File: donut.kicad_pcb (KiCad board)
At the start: 2 copper layers, 78.5 x 68.9 mm, 47 parts, among them J1 AVRISP6, J2 Jack, J3 HALL2, P1 PAD1, P2 PAD2, SW1 S0, SW10 TACTILE, SW11 TACTILE, SW12 TACTILE, SW13 MODE, SW2 TACTILE, SW3 TACTILE, SW4 TACTILE, SW5 TACTILE, SW6 TACTILE, SW7 TACTILE, SW8 TACTILE, SW9 TACTILE, U1 ATMEGA48PA-MU, X1 XTAL4P

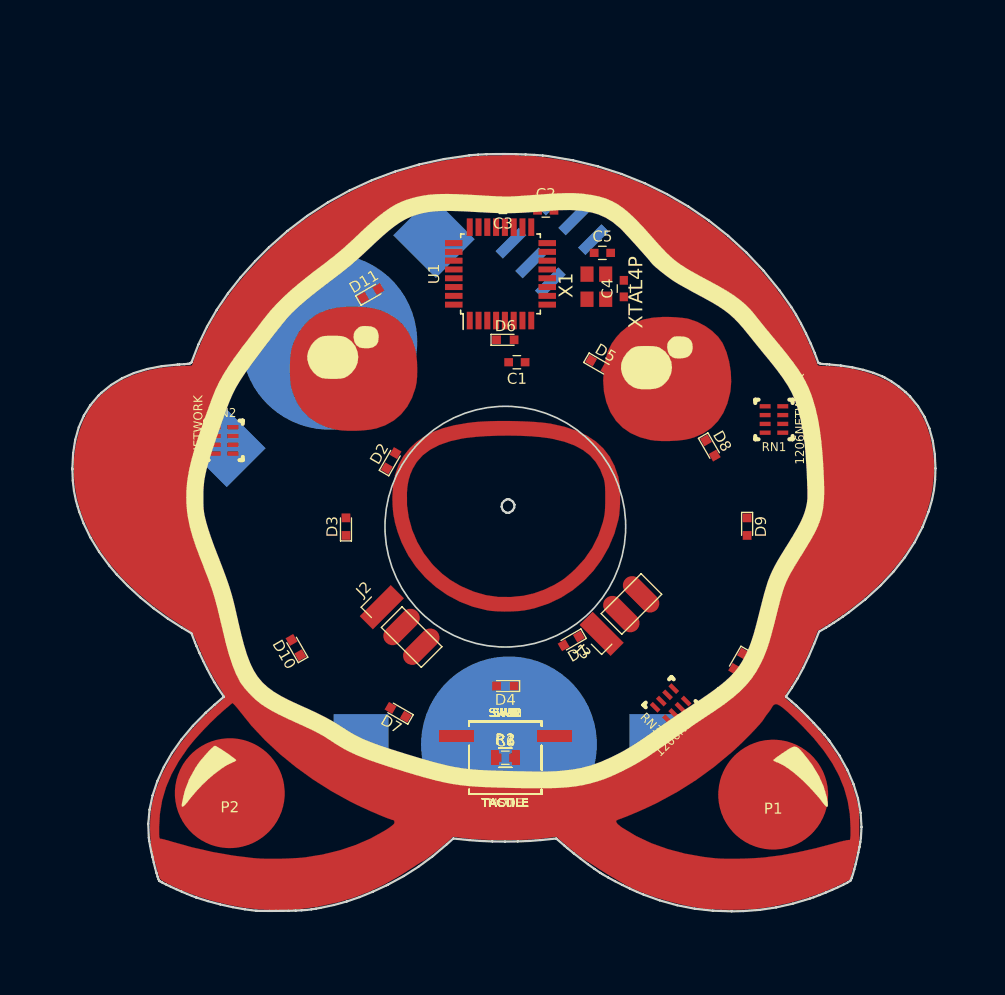
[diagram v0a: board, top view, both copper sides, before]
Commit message: Update donut
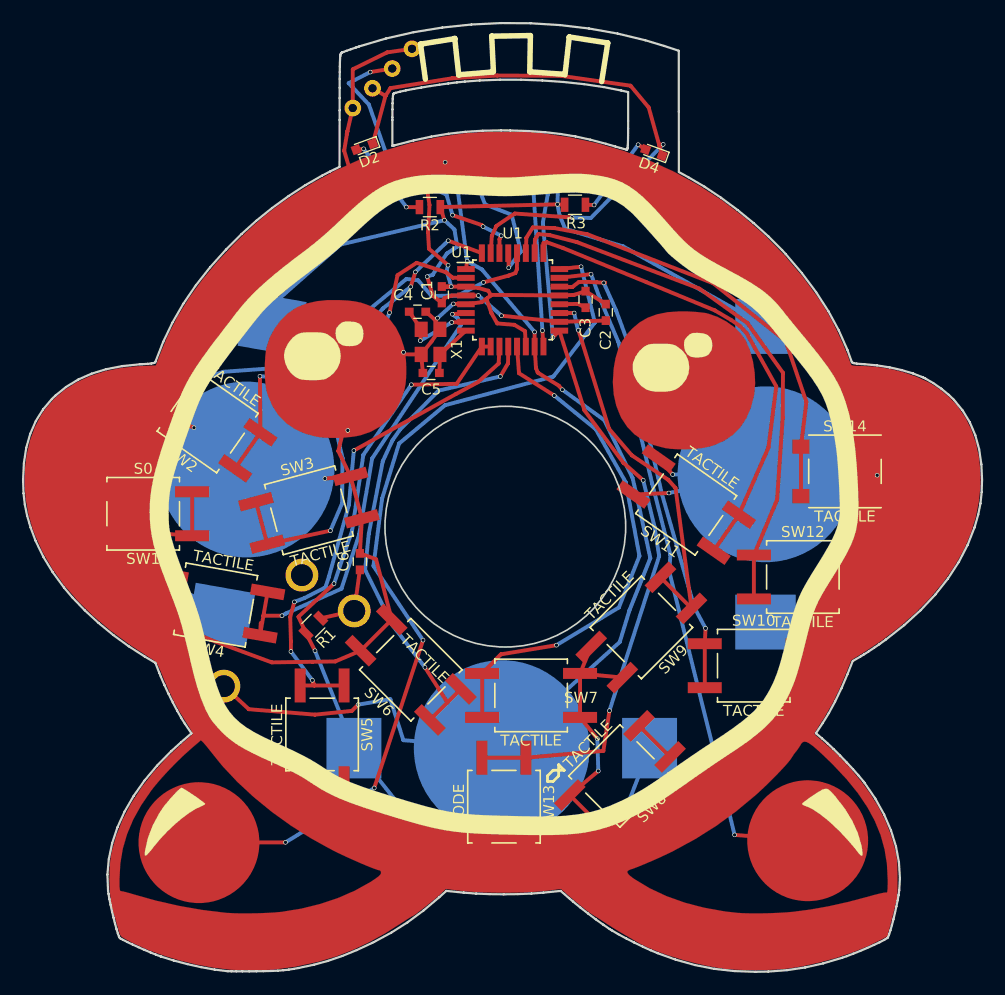
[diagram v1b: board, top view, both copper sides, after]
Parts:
- removed D1, D11, D3, D5, D7, D9: GRN, LED_0603
- removed D10, D12, D6, D8: RED, LED_0603
- removed G***: LOGO, kingdonut:kingdonut2
- removed J3: HALL2, Pin_Header_Straight_1x03_Pitch2.54mm
- removed RN1, RN2, RN3: 1206NETWORK, 1206NETWORK
- added BT2: Battery_Cell, S8211-45R, B.Cu at (-23.6, -5.20)
- added G0: PAD1, kingdonut2, F.Cu at (-0.21, -5.97)
- added P3: PAD2, SMTPIN, F.Cu at (-8.49, -43.5)
- added P4: PAD1, SMTPIN, F.Cu at (-10.3, -41.7)
- added P5: PAD2, SMTPIN, F.Cu at (-12.1, -39.9)
- added P6: PAD2, SMTPIN, F.Cu at (-13.9, -38.1)
- added SW14: TACTILE, TACTILE10Small, F.Cu at (30.9, -5.03)
- C3: value .1uF -> .33uF
- J1: footprint RIBBON6SMT -> RIBBON6SMT_POGO
- J2: footprint Pin_Header_Straight_1x03_Pitch2.54mm -> 3.5mm_barrel_jack_MJ-3536N; moved to B.Cu
- moved R3 50.7 mm to (6.34, -29.3)
- moved R2 50.6 mm to (-6.87, -29.1), turned to 180 degrees
- moved D4 50.4 mm to (13.5, -34.0), turned to 160 degrees
- moved SW2 40.8 mm to (-27.1, -9.49), turned to 145 degrees
- moved LS1 40.2 mm to (-0.33, 20.1), turned to 0 degrees
- moved SW1 39.7 mm to (-33.0, -1.18), turned to 180 degrees
- moved BT1 33.9 mm to (23.7, -4.77), turned to 90 degrees
- moved SW12 31.7 mm to (27.1, 4.58)
- moved SW4 29.8 mm to (-26.4, 7.13), turned to 170 degrees
- moved SW3 28.7 mm to (-17.9, -1.49), turned to 15 degrees
- moved D2 28.7 mm to (-12.8, -34.6), turned to 200 degrees
- moved SW11 28.3 mm to (16.5, -2.00), turned to 145 degrees
- moved SW10 24.1 mm to (22.6, 12.7)
- moved C6 22.2 mm to (-13.2, 3.18), turned to 90 degrees
- moved R1 21.2 mm to (-17.5, 9.01), turned to 225 degrees
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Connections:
- U1 pad 11: TSW9 -> TSW4
- U1 pad 12: TSW7 -> TSW5
- U1 pad 13: TSW5 -> TSW6
- U1 pad 19: TSW10 -> TSW8
- U1 pad 2: TSW6 -> TSW2
- U1 pad 22: TSW11 -> TSW9
- U1 pad 25: TSW0 -> TSW10
- U1 pad 26: TSW1 -> TSW11
- U1 pad 27: TSW2 -> TSW12
- U1 pad 28: TSW3 -> TSW0
- U1 pad 30: (no net) -> RX
- U1 pad 32: TSW4 -> TSW1
- U1 pad 6: VCC -> TSW3
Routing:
- net GND: track 0.00 -> 335.4 mm, vias 0 -> 14
- net VCC: track 0.00 -> 165.8 mm, vias 0 -> 5
- net AUD-: track 0.00 -> 98.7 mm, vias 0 -> 4
- net AUD: track 0.00 -> 81.1 mm, vias 0 -> 3
- net Net-(P2-Pad1): track 0.00 -> 80.1 mm, vias 0 -> 4
- net SCK: track 0.00 -> 72.9 mm, vias 0 -> 3
- net Net-(P1-Pad1): track 0.00 -> 62.4 mm, vias 0 -> 2
- net TSW0: track 0.00 -> 57.9 mm, vias 0 -> 2
- net TX: track 0.00 -> 57.1 mm, vias 0 -> 2
- net TSW11: track 0.00 -> 49.3 mm
- net TSW6: track 0.00 -> 46.7 mm, vias 0 -> 2
- net TSW5: track 0.00 -> 45.2 mm, vias 0 -> 2
- net TSW4: track 0.00 -> 45.2 mm, vias 0 -> 4
- net TSW2: track 0.00 -> 43.4 mm, vias 0 -> 2
- net TSW10: track 0.00 -> 43.1 mm
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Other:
- board size 78.5 x 68.9 mm -> 87.3 x 86.3 mm

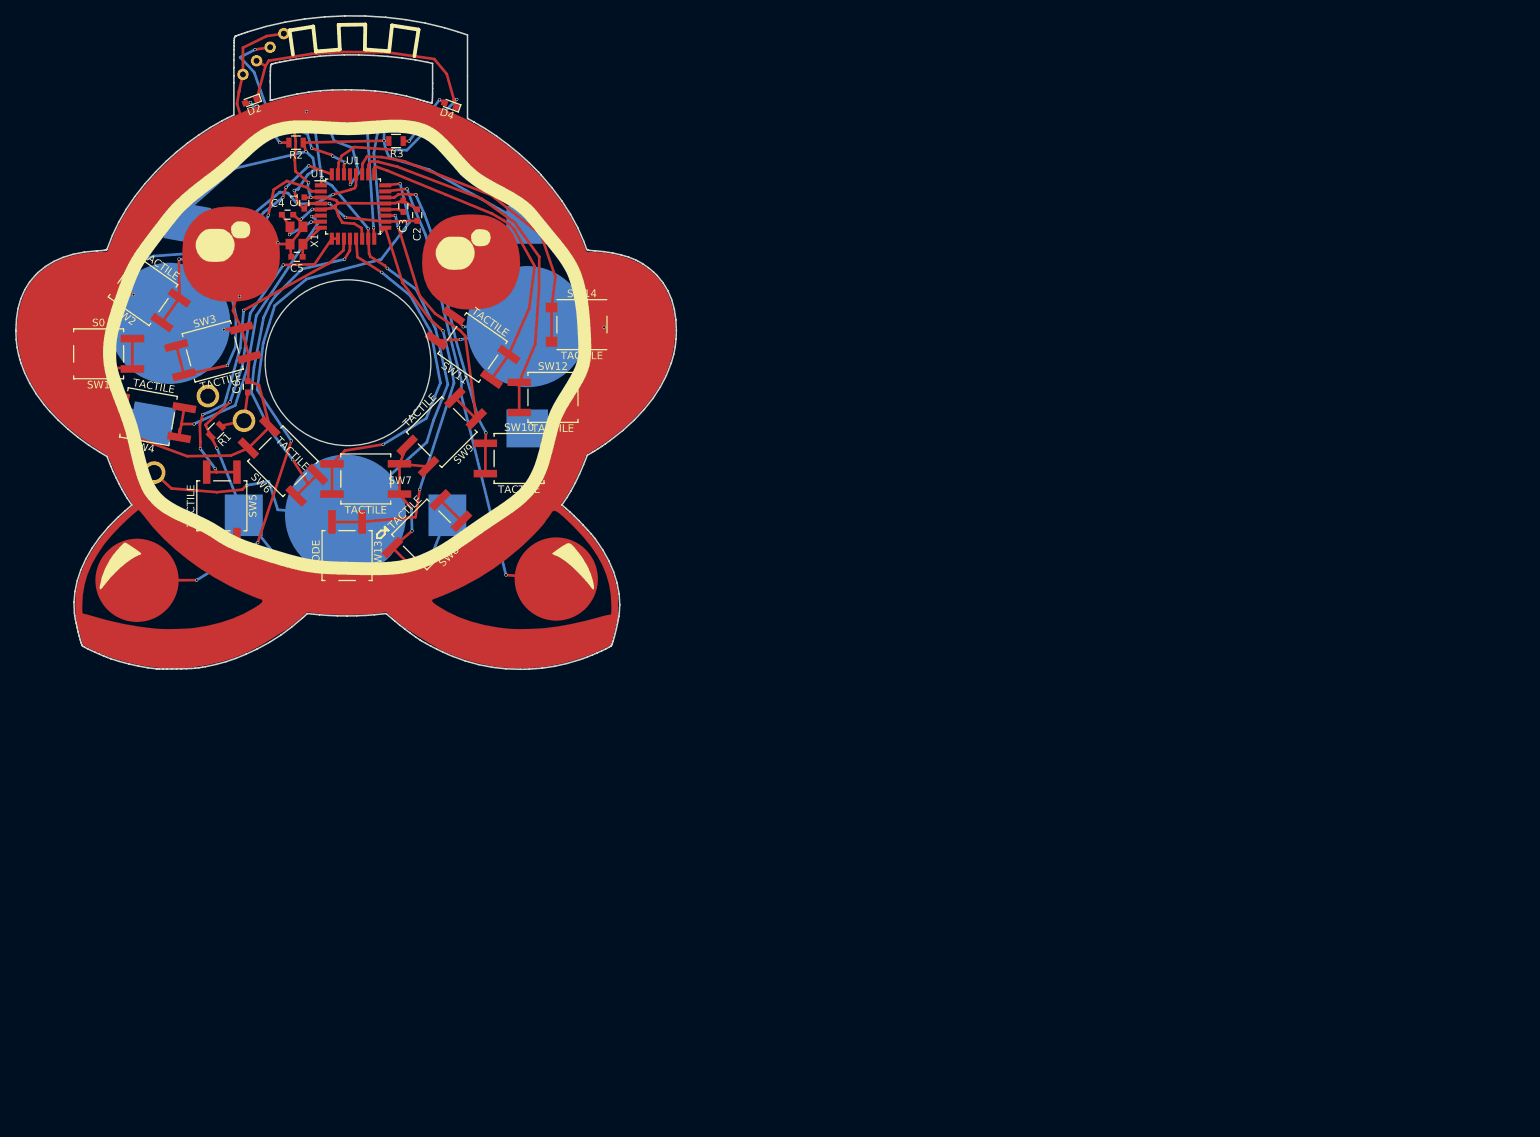
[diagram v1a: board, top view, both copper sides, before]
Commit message: Update
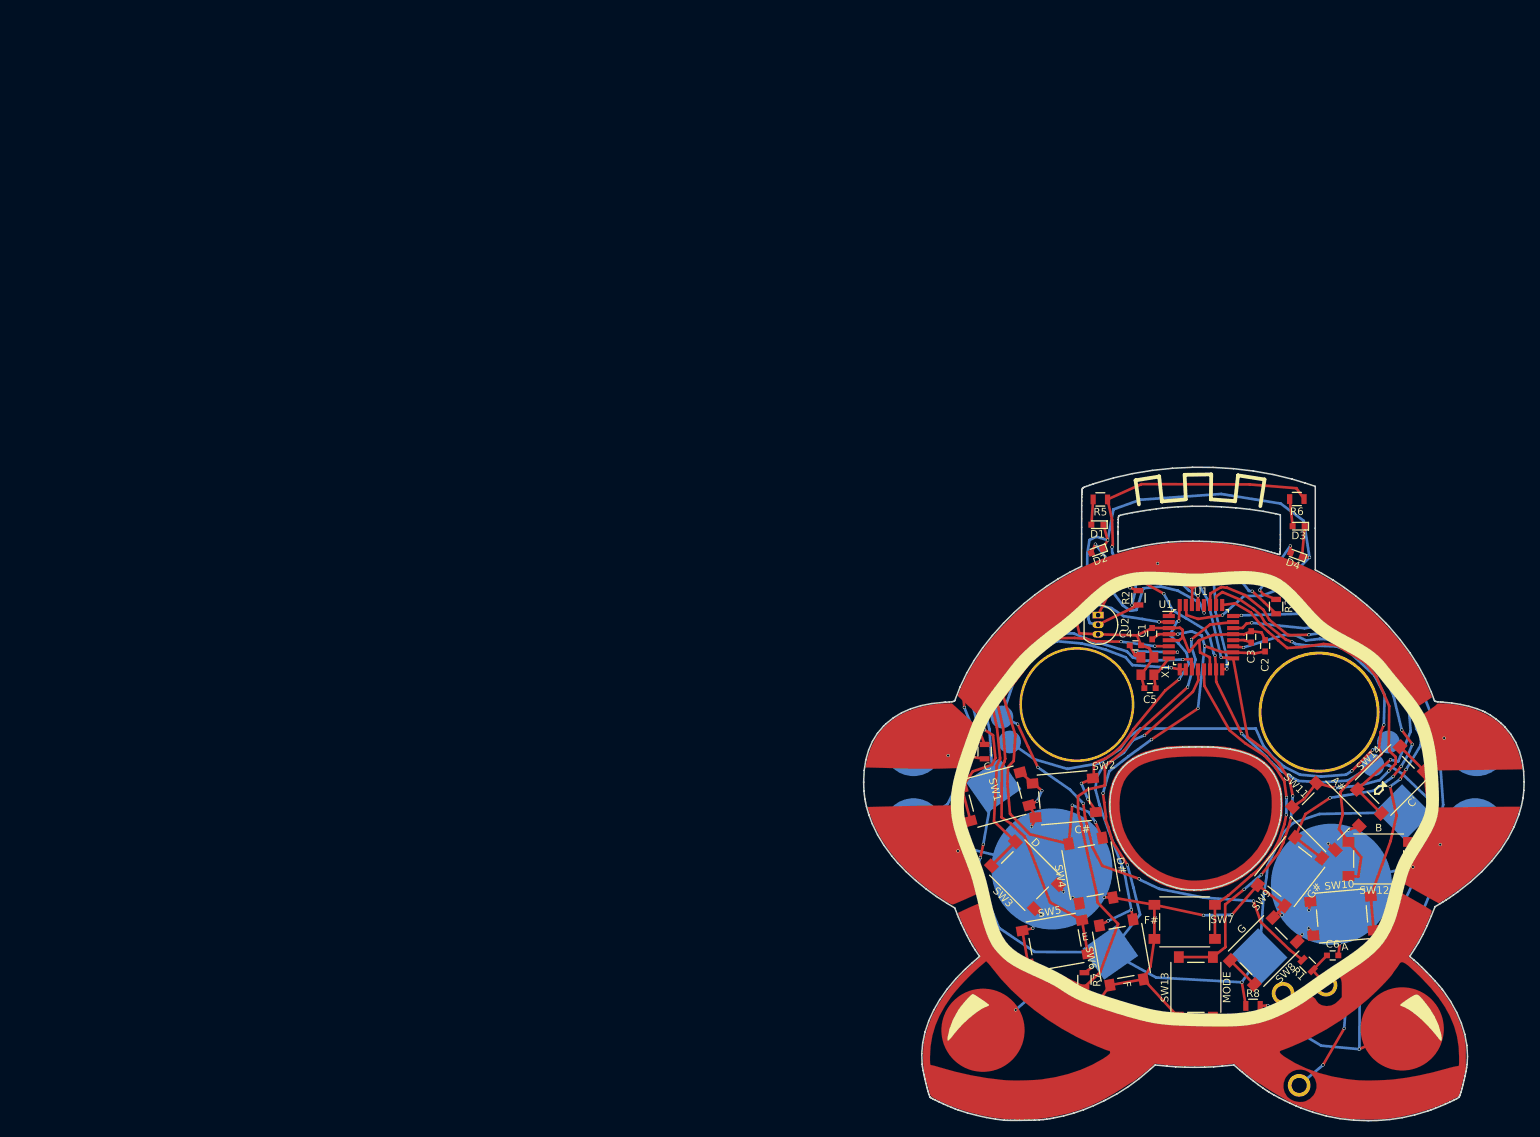
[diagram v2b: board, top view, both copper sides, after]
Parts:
- removed LS1: Speaker, S8211-45R
- added D1: NP, LED_0603, F.Cu at (99.0, 21.4)
- added D3: NP, LED_0603, F.Cu at (125.6, 21.6)
- added P10: PAD2, SMTPIN, F.Cu at (149.1, 62.0)
- added P11: PAD2, SMTPIN, B.Cu at (137.4, 50.1)
- added P12: PAD2, SMTPIN, B.Cu at (86.4, 46.8)
- added P13: PAD2, SMTPIN, B.Cu at (87.4, 50.1)
- added P14: PAD2, SMTPIN, B.Cu at (135.4, 53.2)
- added P7: PAD2, SMTPIN, B.Cu at (74.7, 50.6)
- added P8: PAD1, SMTPIN, B.Cu at (149.1, 50.6)
- added P9: PAD2, SMTPIN, B.Cu at (148.9, 61.5)
- added R4: 560, R_0805, F.Cu at (84.1, 51.4)
- added R5: NP, R_0805, F.Cu at (99.4, 18.1)
- added R6: NP, R_0805, F.Cu at (125.3, 18.0)
- added R7: 470k, R_0805, F.Cu at (97.3, 81.5)
- added R8: 470k, R_0805, F.Cu at (119.6, 85.0)
- added U2: TSDP343xx, TO-92_Inline_Narrow_Oval, F.Cu at (99.1, 33.3)
- P3: moved to B.Cu
- R2, R3: value 1k -> 560
- SW1: value S0 -> C; footprint TACTILE10 -> TACTILE10Small
- SW10: value TACTILE -> A; footprint TACTILE10 -> TACTILE10Small
- SW11: value TACTILE -> A#; footprint TACTILE10 -> TACTILE10Small
- SW12: value TACTILE -> B; footprint TACTILE10 -> TACTILE10Small
- SW13: footprint TACTILE10 -> TACTILE10Small
- SW14: value TACTILE -> C'
- SW2: value TACTILE -> C#; footprint TACTILE10 -> TACTILE10Small
- SW3: value TACTILE -> D; footprint TACTILE10 -> TACTILE10Small
- SW4: value TACTILE -> D#; footprint TACTILE10 -> TACTILE10Small
- SW5: value TACTILE -> E; footprint TACTILE10 -> TACTILE10Small
- SW6: value TACTILE -> F; footprint TACTILE10 -> TACTILE10Small
- SW7: value TACTILE -> F#; footprint TACTILE10 -> TACTILE10Small
- SW8: value TACTILE -> G; footprint TACTILE10 -> TACTILE10Small
- SW9: value TACTILE -> G#; footprint TACTILE10 -> TACTILE10Small
- moved P4 183.8 mm to (148.6, 50.6)
- moved J2 163.1 mm to (128.6, 84.6), turned to 75 degrees
- moved C6 161.8 mm to (130.1, 78.3), turned to 0 degrees
- moved R1 160.6 mm to (126.8, 79.6), turned to 135 degrees
- moved P6 139.0 mm to (78.8, 65.6)
- moved SW2 138.9 mm to (94.6, 57.5), turned to 5 degrees
- moved SW4 138.2 mm to (98.1, 67.1), turned to 100 degrees
- moved BT2 137.0 mm to (93.0, 66.9), turned to 305 degrees
- moved P3 134.0 mm to (74.7, 61.5), turned to 135 degrees
- moved SW1 132.1 mm to (85.5, 57.3), turned to 195 degrees
- moved R3 131.5 mm to (122.6, 32.2), turned to 90 degrees
- moved P5 129.3 mm to (79.3, 51.6)
- moved BT1 129.3 mm to (129.9, 68.9), turned to 45 degrees
- moved SW11 128.6 mm to (129.2, 59.9), turned to 135 degrees
- moved SW6 128.4 mm to (102.2, 77.9), turned to 100 degrees
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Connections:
- P1 pad 1: Net-(P1-Pad1) -> TOUCH2
- P2 pad 1: Net-(P2-Pad1) -> TOUCH1
- P5 pad 1: TX -> Net-(P5-Pad1)
- SW1 pad 1: TSW0 -> GND
- SW1 pad 2: TSW0 -> GND
- SW1 pad 3: GND -> TSW0
- SW1 pad 4: GND -> TSW0
- SW10 pad 1: TSW9 -> GND
- SW10 pad 2: TSW9 -> GND
- SW10 pad 3: GND -> TSW9
- SW10 pad 4: GND -> TSW9
- SW11 pad 1: TSW10 -> GND
- SW11 pad 2: TSW10 -> GND
- SW11 pad 3: GND -> TSW10
- SW11 pad 4: GND -> TSW10
- SW12 pad 1: TSW11 -> GND
- SW12 pad 2: TSW11 -> GND
- SW12 pad 3: GND -> TSW11
- SW12 pad 4: GND -> TSW11
- SW13 pad 1: SCK -> GND
- SW13 pad 2: SCK -> GND
- SW13 pad 3: GND -> SCK
- SW13 pad 4: GND -> SCK
- SW2 pad 1: TSW1 -> GND
- SW2 pad 2: TSW1 -> GND
- SW2 pad 3: GND -> TSW1
- SW2 pad 4: GND -> TSW1
- SW3 pad 1: TSW2 -> GND
- SW3 pad 2: TSW2 -> GND
- SW3 pad 3: GND -> TSW2
- SW3 pad 4: GND -> TSW2
- SW4 pad 1: TSW3 -> GND
- SW4 pad 2: TSW3 -> GND
- SW4 pad 3: GND -> TSW3
- SW4 pad 4: GND -> TSW3
- SW5 pad 1: TSW4 -> GND
- SW5 pad 2: TSW4 -> GND
- SW5 pad 3: GND -> TSW4
- SW5 pad 4: GND -> TSW4
- SW6 pad 1: TSW5 -> GND
- SW6 pad 2: TSW5 -> GND
- SW6 pad 3: GND -> TSW5
- SW6 pad 4: GND -> TSW5
- SW7 pad 1: TSW6 -> GND
- SW7 pad 2: TSW6 -> GND
- SW7 pad 3: GND -> TSW6
- SW7 pad 4: GND -> TSW6
- SW8 pad 1: TSW7 -> GND
- SW8 pad 2: TSW7 -> GND
- SW8 pad 3: GND -> TSW7
- SW8 pad 4: GND -> TSW7
- SW9 pad 1: TSW8 -> GND
- SW9 pad 2: TSW8 -> GND
- SW9 pad 3: GND -> TSW8
- SW9 pad 4: GND -> TSW8
- U1 pad 23: Net-(P1-Pad1) -> TOUCH1
- U1 pad 24: Net-(P2-Pad1) -> TOUCH2
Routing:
- net VCC: track 165.8 -> 272.9 mm, vias 5 -> 13
- net TOUCH2: track 0.00 -> 103.1 mm, vias 0 -> 3
- net Net-(P2-Pad1): track 80.1 -> 0.00 mm, vias 4 -> 0
- net TOUCH1: track 0.00 -> 78.9 mm, vias 0 -> 4
- net Net-(P1-Pad1): track 62.4 -> 0.00 mm, vias 2 -> 0
- net Net-(P11-Pad1): track 0.00 -> 57.2 mm, vias 0 -> 2
- net TX: track 57.1 -> 100.8 mm, vias 2 -> 4
- net RX: track 26.8 -> 67.4 mm, vias 4 -> 1
- net TSW4: track 45.2 -> 71.2 mm, vias 4 -> 2
- net TSW8: track 35.6 -> 58.1 mm, vias 2 -> 6
- net TSW3: track 42.1 -> 61.8 mm, vias 2 -> 4
- net TSW9: track 42.7 -> 62.3 mm, vias 2 -> 4
- net GND: track 335.4 -> 350.2 mm, vias 14 -> 22
- net TSW12: track 42.7 -> 55.0 mm, vias 0 -> 2
- net TSW2: track 43.4 -> 54.9 mm, vias 2 -> 4
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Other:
- outline, holes or cut-outs redrawn
- board text added: "USE ONLY BATTERIES OF SIMILAR CHARGE"
- board text removed: "80mm x 80mm - artwork should be 944 px wide."
